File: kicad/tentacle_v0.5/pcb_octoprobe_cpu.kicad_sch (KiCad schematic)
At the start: 27 parts, among them J201 Conn_02x05, U201 RP2040, U203 W25Q32JVS, X201 Oscillator-12MHz

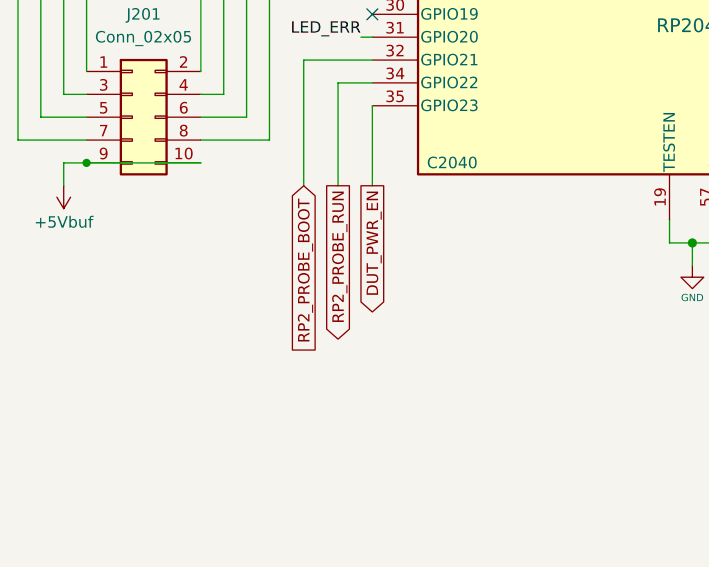
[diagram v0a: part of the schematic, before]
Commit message: tentacle v0.5 kicad - unknown small changes to schematics
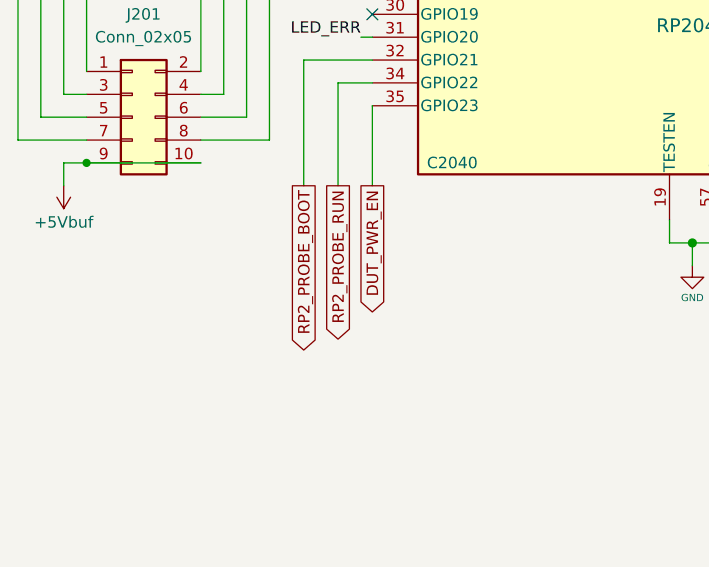
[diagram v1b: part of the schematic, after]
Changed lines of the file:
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@@
 	)
 	(global_label "RP2_PROBE_BOOT"
-		(shape input)
+		(shape output)
 		(at 45.72 115.57 270)
 		(fields_autoplaced yes)
